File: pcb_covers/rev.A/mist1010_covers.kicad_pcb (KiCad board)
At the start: 2 copper layers, 133.5 x 61.5 mm, 1 part

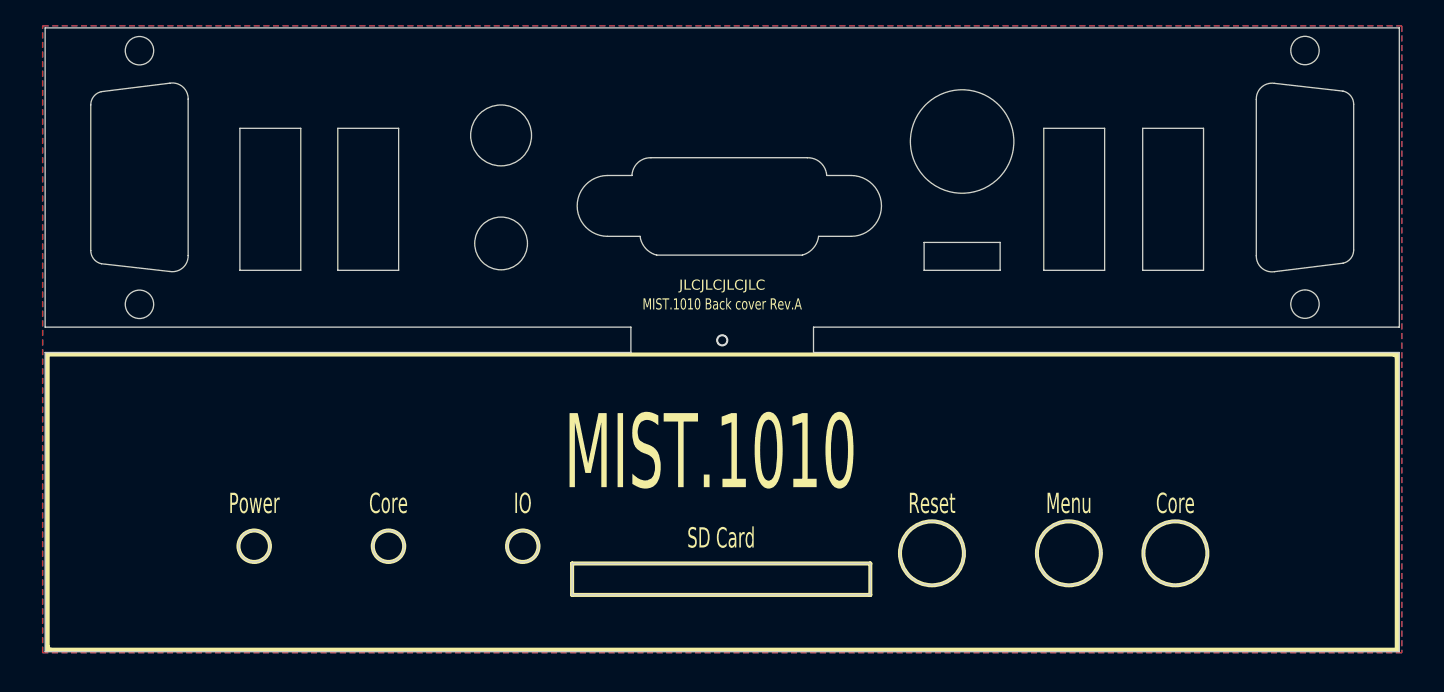
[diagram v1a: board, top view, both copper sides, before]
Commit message: update pcb rev.A
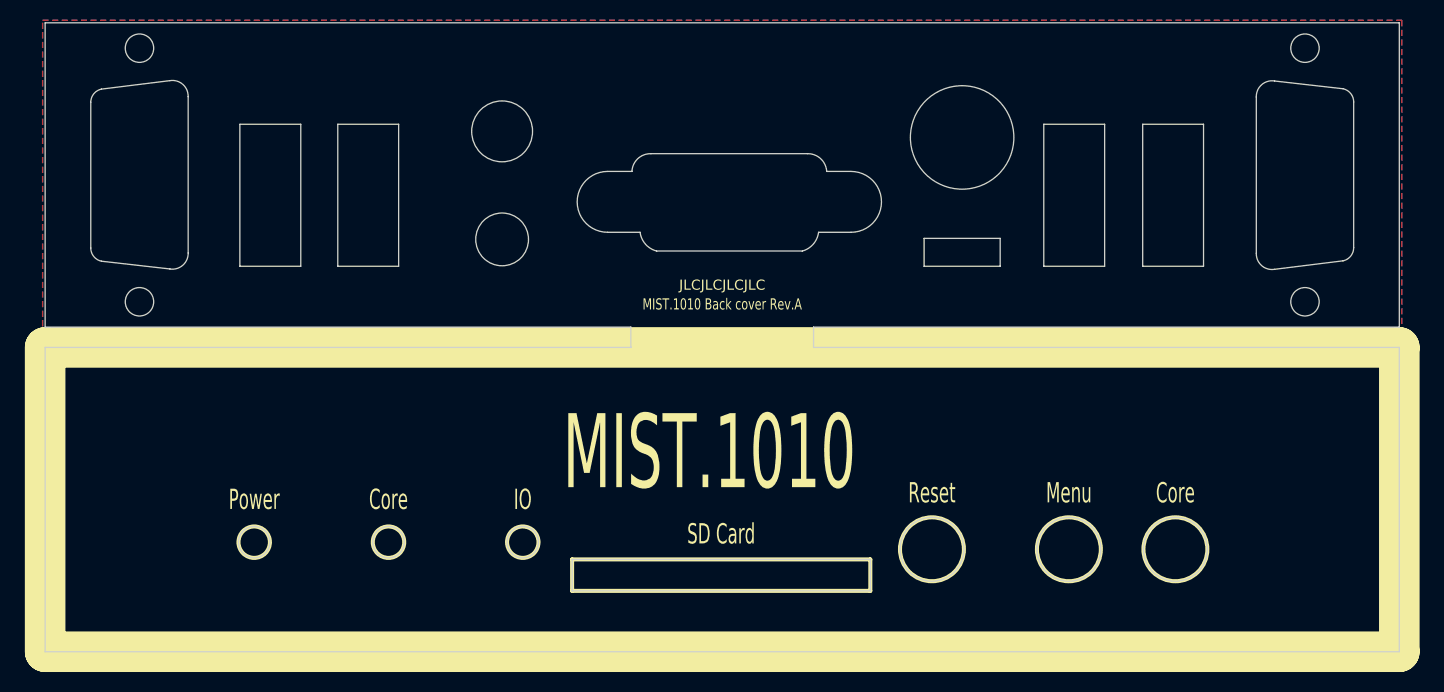
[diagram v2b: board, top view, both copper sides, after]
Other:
- board size 133.5 x 61.5 mm -> 133.5 x 62 mm

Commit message: update pcb rev.A
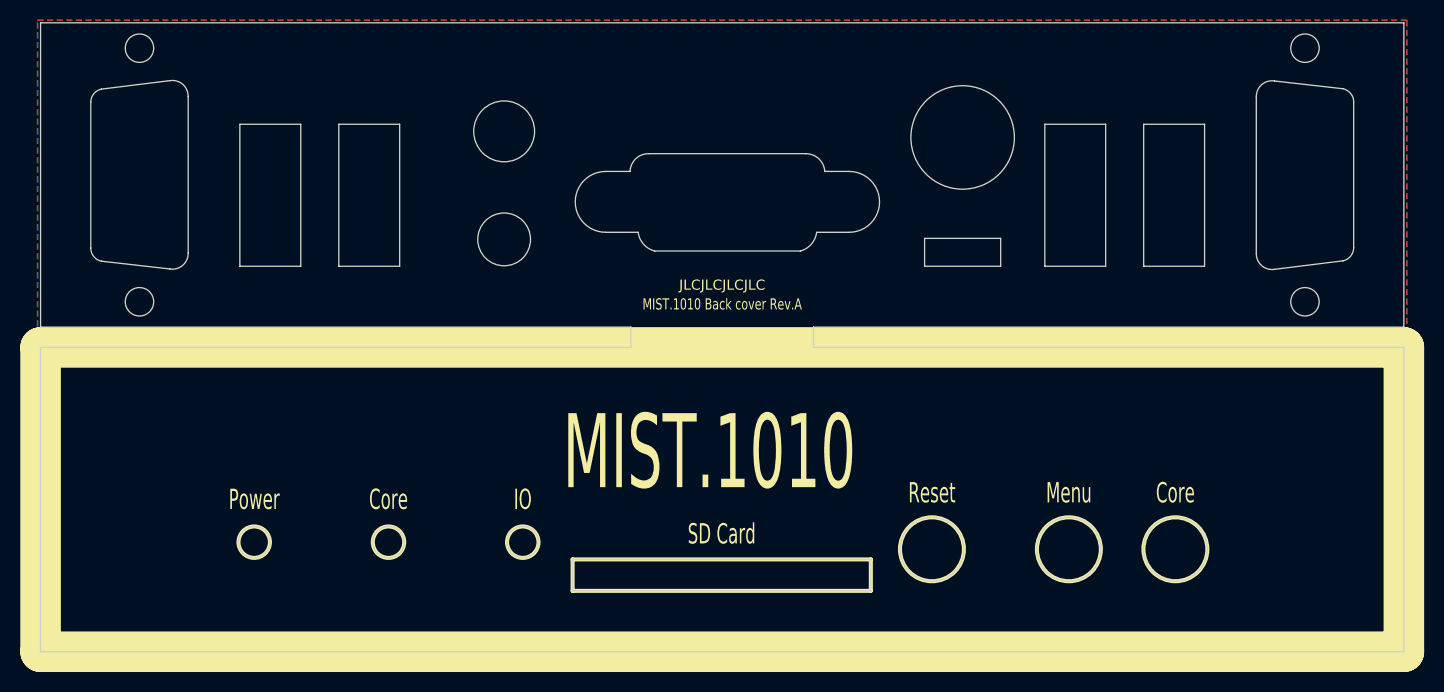
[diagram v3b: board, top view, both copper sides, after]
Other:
- board size 133.5 x 62 mm -> 134.4 x 62 mm
